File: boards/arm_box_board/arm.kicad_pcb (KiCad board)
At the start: 2 copper layers, 5 parts, among them J1 Output, J2 24V, U1 Teensy4.1, U2 PololuD24V5F5, U3 TMC2209_SILENTSTEPSTICK

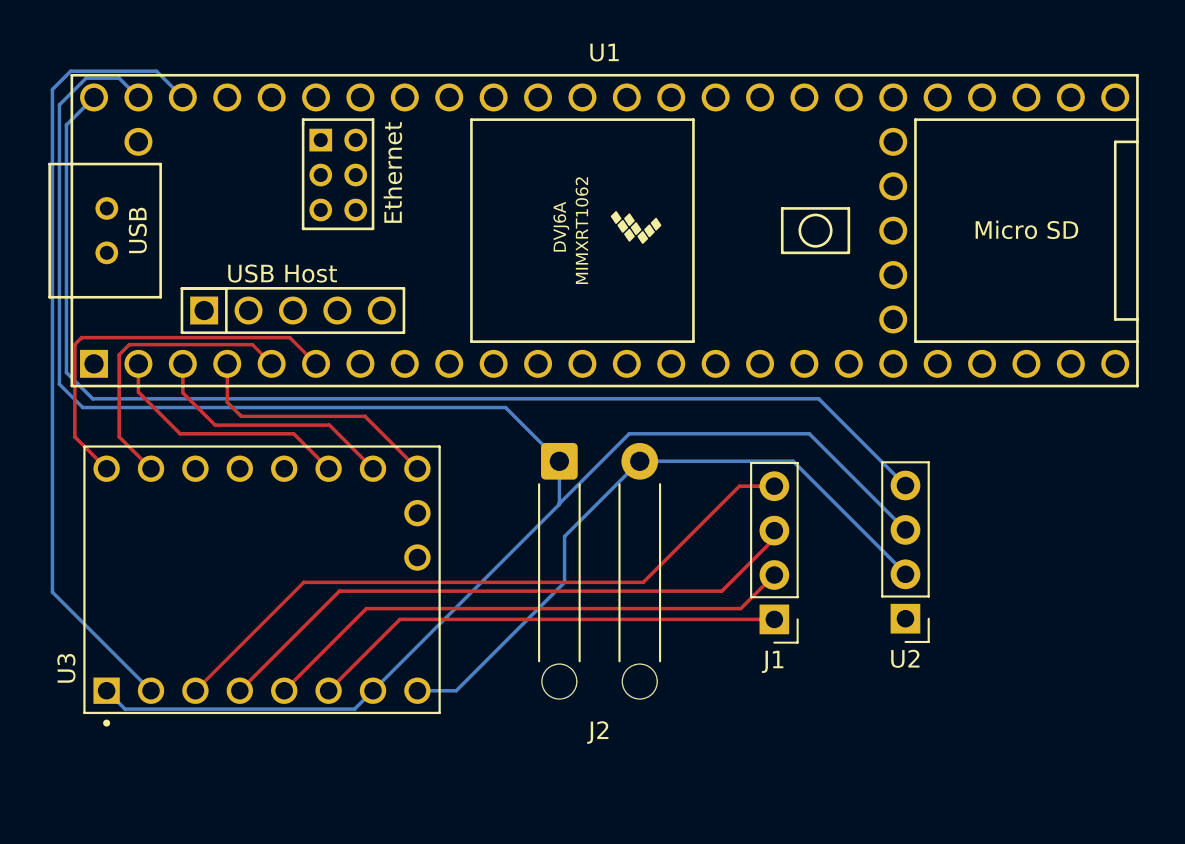
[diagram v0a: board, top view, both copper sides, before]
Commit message: Updated Arm board with ethernet
updated on 04/24
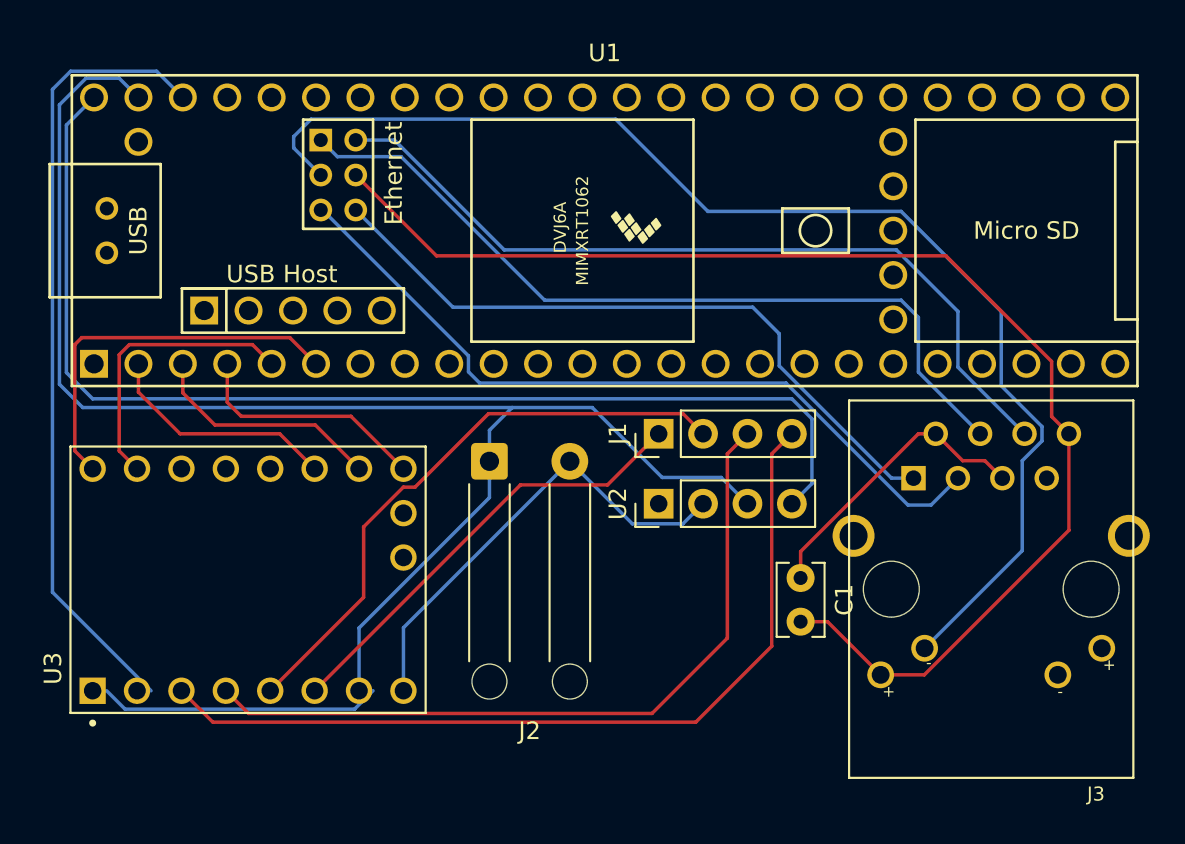
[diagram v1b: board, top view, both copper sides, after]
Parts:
- added C1: C_Small, Capacitor_THT:C_Rect_L4.0mm_W2.5mm_P2.50mm, F.Cu at (116.5, 100.8)
- added J3: J00-0045NL, EthernetConn:PULSE_J00-0045NL, F.Cu at (127.4, 101.4)
- moved U2 15.6 mm to (108.4, 96.5), turned to 90 degrees
- moved J1 12.5 mm to (108.4, 92.5), turned to 90 degrees
- moved J2 4.00 mm to (98.7, 94.1)
- moved U3 0.80 mm to (84.9, 100.8)
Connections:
- U1 pad 60: unconnected-(U1-R+-Pad60) -> Net-(J3-CTT)
- U1 pad 61: unconnected-(U1-LED-Pad61) -> Net-(J3-LC)
- U1 pad 62: unconnected-(U1-T--Pad62) -> Net-(J3-RD+)
- U1 pad 63: unconnected-(U1-T+-Pad63) -> Net-(J3-TD+)
- U1 pad 64: unconnected-(U1-GND-Pad64) -> Net-(J3-GND)
- U1 pad 65: unconnected-(U1-R--Pad65) -> Net-(J3-RD-)
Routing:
- net Net-(J3-GND): track 0.00 -> 74.3 mm
- net Net-(J3-LC): track 0.00 -> 71.3 mm
- net Net-(J3-RD-): track 0.00 -> 47.1 mm
- net Net-(J3-CTT): track 0.00 -> 46.5 mm
- net Net-(J3-RD+): track 0.00 -> 44.6 mm
- net Net-(J3-TD+): track 0.00 -> 39.3 mm
- net Net-(J3-CTR): track 0.00 -> 16.9 mm
- net Net-(J2-Pin_2): track 37.9 -> 26.6 mm
- net Net-(J1-Pin_4): track 38.0 -> 48.9 mm
- net Net-(J2-Pin_1): track 109.4 -> 99.7 mm
- net Net-(J1-Pin_3): track 34.6 -> 43.2 mm
- net Net-(J1-Pin_2): track 30.8 -> 34.2 mm
- net Net-(U1-VIN): track 67.1 -> 65.5 mm
- net Net-(J1-Pin_1): track 27.2 -> 25.8 mm
- net Net-(U1-1_TX1_CTX2_MISO1): track 14.3 -> 13.5 mm
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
